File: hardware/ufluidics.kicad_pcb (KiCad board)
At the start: 2 copper layers, 93.4 x 77.8 mm, 79 parts, among them J1 Conn_01x08, J10 Conn_01x08, J11 Conn_01x08, J12 Conn_01x04, J13 Conn_01x08, J14 Conn_01x08, J15 Conn_01x04, J16 Conn_01x03, J17 Conn_01x03, J2 Conn_01x08, J22 Connector, USB-TYPE-C-16P, J3 Conn_01x04, J4 Conn_01x08, J5 Conn_01x08, J6 Conn_01x04, J7 Conn_01x08, J8 Conn_01x08, J9 Conn_01x04, Q1 SUD50P06-15, U1 ESP32-S3-WROOM-1, U3 AP7361C-33E, U5 LM2675M-5

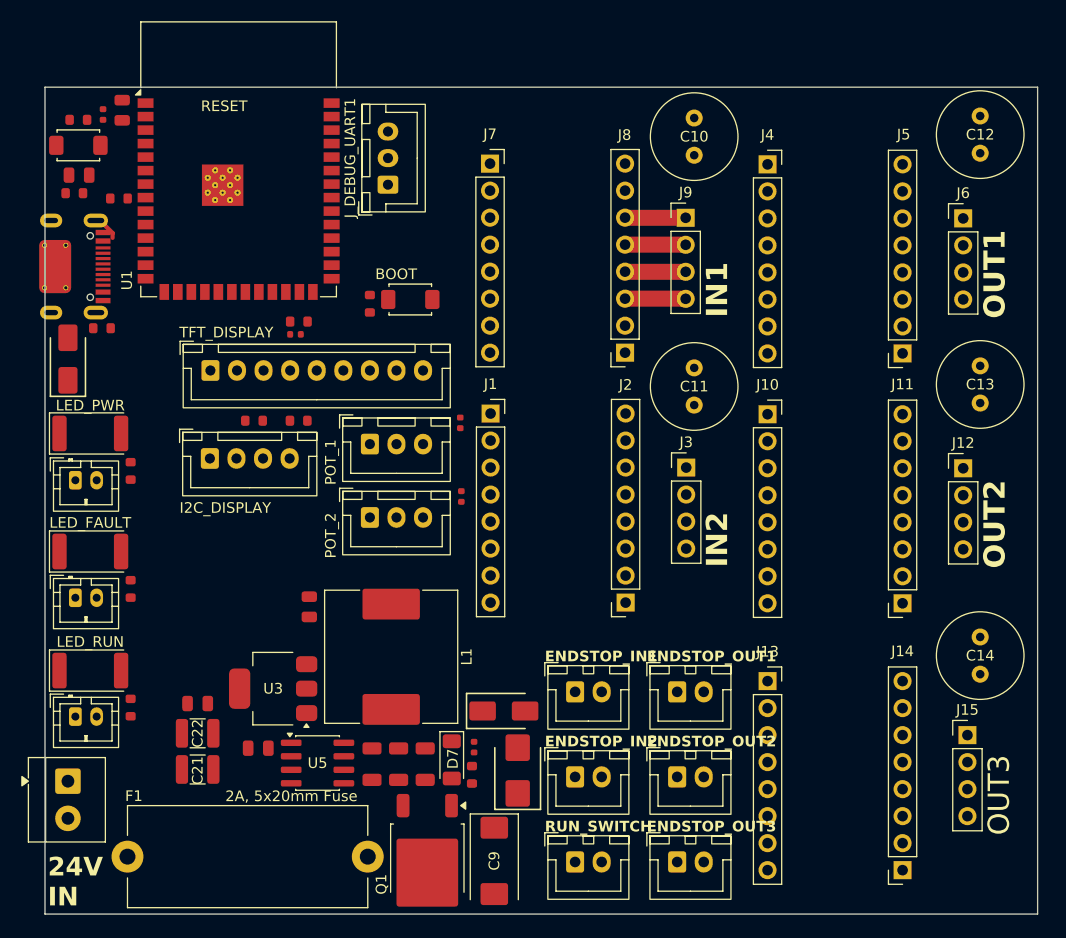
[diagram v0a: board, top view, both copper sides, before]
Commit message: route
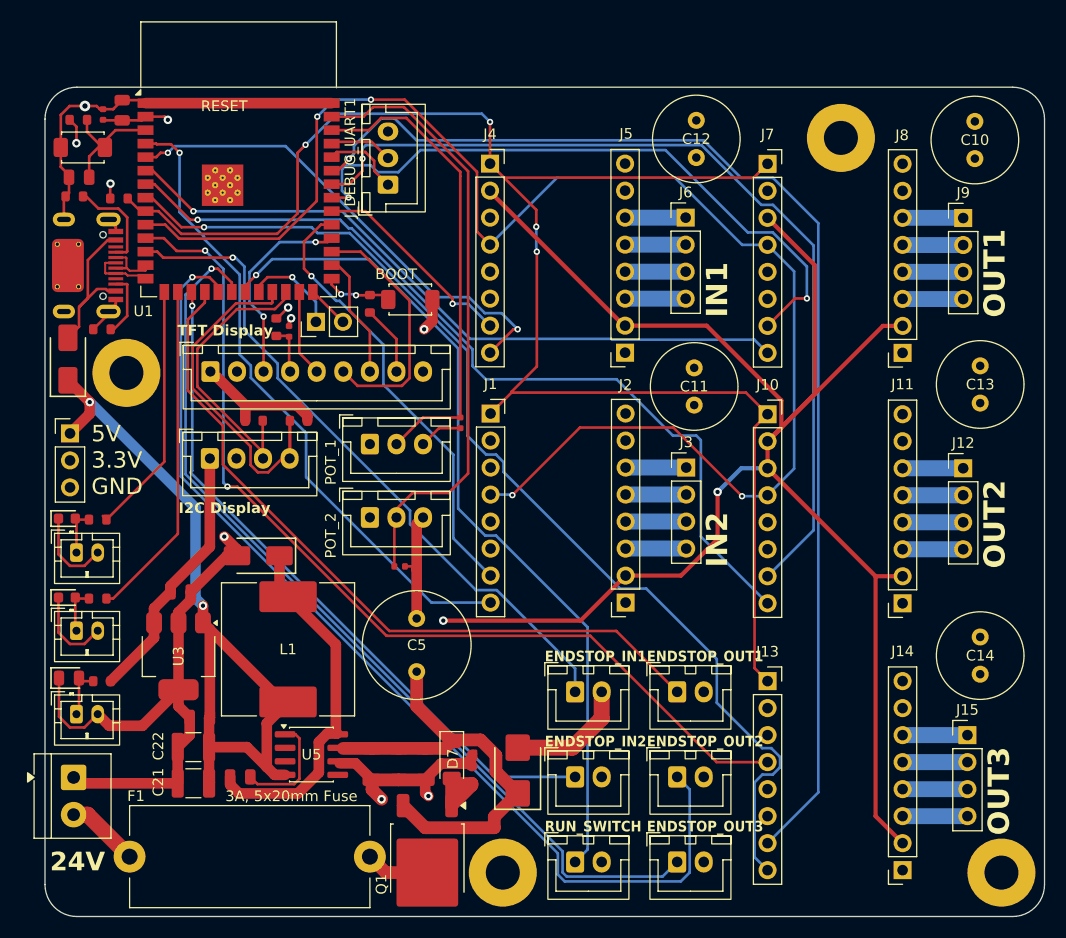
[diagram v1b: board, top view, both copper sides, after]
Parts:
- removed C9: 470uF, Capacitor_Tantalum_SMD:CP_EIA-7343-31_Kemet-D
- removed LED_FAULT, LED_PWR, LED_RUN: LED, LED_SMD:LED_2512_6332Metric
- removed R4: 1k, PCM_JLCPCB:R_0603
- added C5: 470 uF 35V, Capacitor_THT:C_Radial_D10.0mm_H16.0mm_P5.00mm, F.Cu at (134.7, 102.9)
- added D1: Green, PCM_JLCPCB:D_0805, F.Cu at (102.0, 103.5)
- added D3: Red, PCM_JLCPCB:D_0603, F.Cu at (101.8, 95.9)
- added D5: Yellow, PCM_JLCPCB:D_0603, F.Cu at (101.8, 88.5)
- added J18: Conn_01x03, Connector_PinHeader_2.54mm:PinHeader_1x03_P2.54mm_Vertical, F.Cu at (102.1, 80.5)
- added J21: Conn_01x02, Connector_PinHeader_2.54mm:PinHeader_1x02_P2.54mm_Vertical, F.Cu at (125.2, 70.0)
- added R10: 1kΩ, PCM_JLCPCB:R_0603, F.Cu at (104.7, 88.6)
- added REF**: MountingHole_3.2mm_M3_Pad, MountingHole:MountingHole_3.2mm_M3_Pad, F.Cu at (189.7, 121.8)
- added REF**: MountingHole_3.2mm_M3_Pad, MountingHole:MountingHole_3.2mm_M3_Pad, F.Cu at (174.6, 52.7)
- added REF**: MountingHole_3.2mm_M3_Pad, MountingHole:MountingHole_3.2mm_M3_Pad, F.Cu at (142.8, 121.8)
- added REF**: MountingHole_3.2mm_M3_Pad, MountingHole:MountingHole_3.2mm_M3_Pad, F.Cu at (107.4, 74.8)
- R5: value 1k -> 1kΩ
- R6: value 2.2k -> 2.2kΩ
- moved D2 27.3 mm to (119.8, 92.0), turned to 180 degrees
- moved C12 26.7 mm to (161.0, 51.0)
- moved C10 26.4 mm to (187.2, 51.1)
- moved J4 26.1 mm to (141.6, 55.1)
- moved J5 26.1 mm to (154.3, 72.9)
- moved J6 26.1 mm to (160.0, 60.2)
- moved J7 26.1 mm to (167.7, 55.1)
- moved J8 26.1 mm to (180.4, 72.9)
- moved J9 26.1 mm to (186.1, 60.2)
- moved J_LED_PWR1 22.0 mm to (102.7, 106.9)
- moved R6 20.0 mm to (105.1, 103.8), turned to 180 degrees
- moved J_LED_RUN1 15.4 mm to (102.7, 91.7)
- moved C8 12.2 mm to (112.5, 95.4), turned to 0 degrees
- moved L1 9.73 mm to (122.6, 100.8)
- moved U3 9.41 mm to (112.3, 101.5), turned to -90 degrees
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- renumbered I2C_DISPLAY to J19, TFT_DISPLAY to J20
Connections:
- U1 pad 15: unconnected-(U1-IO3-Pad15) -> /LED_RUN
- U1 pad 22: unconnected-(U1-IO14-Pad22) -> /GPIO14
- U1 pad 26: /LED_RUN -> /GPIO45
- U1 pad 38: /POT_B -> /POT_A
- U1 pad 39: /POT_A -> /POT_B
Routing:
- net +3V3: track 0.00 -> 222.8 mm, vias 0 -> 6
- net GND: track 1.41 -> 164.1 mm, vias 0 -> 6
- net DRIVER_EN: track 0.00 -> 151.2 mm, vias 0 -> 4
- net /TMC_UART_A: track 0.00 -> 140.3 mm, vias 0 -> 4
- net /OUT3_STEP: track 0.00 -> 112.8 mm, vias 0 -> 1
- net /OUT3_DIR: track 0.00 -> 101.8 mm, vias 0 -> 1
- net /OUT2_ENDSTOP: track 0.00 -> 97.2 mm, vias 0 -> 1
- net /TMC_UART_B: track 0.00 -> 90.7 mm, vias 0 -> 2
- net /OUT3_ENDSTOP: track 0.00 -> 87.3 mm, vias 0 -> 1
- net /OUT2_STEP: track 0.00 -> 84.9 mm, vias 0 -> 1
- net /OUT2_DIR: track 0.00 -> 81.1 mm, vias 0 -> 1
- net /RUN_SWITCH: track 0.00 -> 79.5 mm, vias 0 -> 1
- net +5V: track 0.00 -> 73.5 mm, vias 0 -> 2
- net /OUT1_ENDSTOP: track 0.00 -> 69.8 mm
- net /OUT1_DIR: track 0.00 -> 65.6 mm, vias 0 -> 1
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- added copper zone on In1.Cu, net +24V
- added copper zone on In1.Cu, net +3V3
- added copper zone on In2.Cu, net GND
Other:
- board size 93.4 x 77.8 mm -> 94 x 78 mm
- copper layers 2 -> 4
- board text added: "24V"
- board text added: "3A, 5x20mm Fuse"
- board text added: "5V 3.3V GND"
- board text added: "I2C Display"
- board text added: "TFT Display"
- board text added: "digital fabrication lab daniel xu 2026"
- board text removed: "24V IN"
- board text removed: "2A, 5x20mm Fuse"
